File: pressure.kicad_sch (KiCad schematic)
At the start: 7 parts, among them IC1 HSFPAR004A, U6 INA317IDGKR

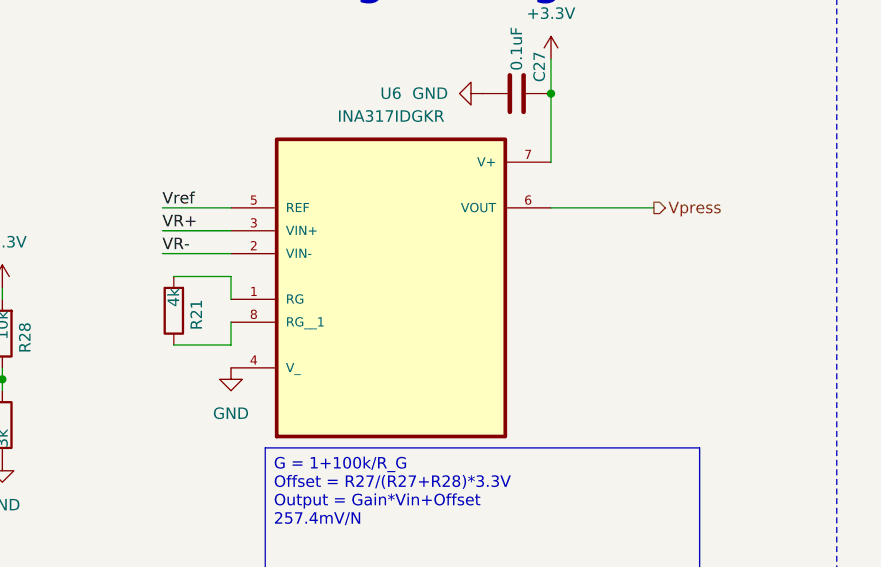
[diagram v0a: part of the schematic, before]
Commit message: further work
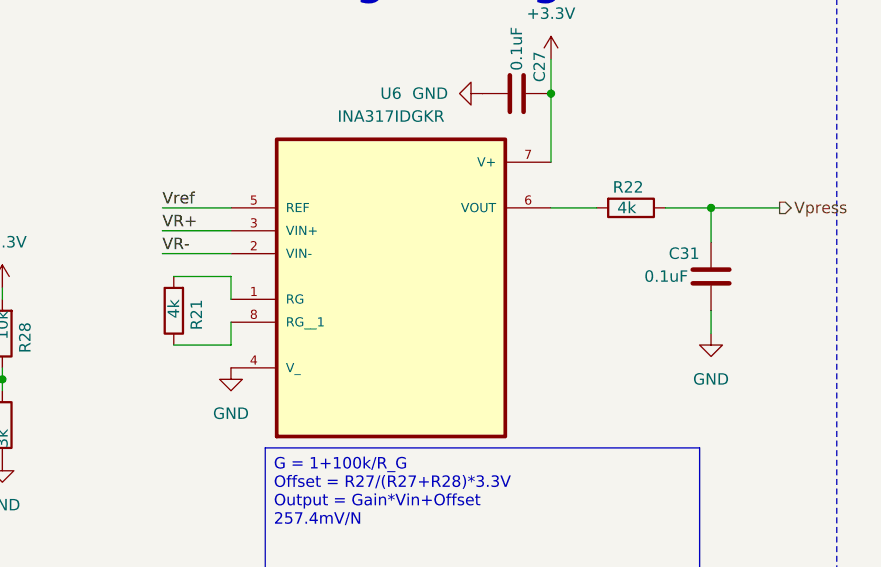
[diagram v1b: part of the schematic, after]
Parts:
- added C31: 0.1uF, Capacitor_SMD:C_0603_1608Metric, symbol Device:C
- added R22: 4k, Resistor_SMD:R_0603_1608Metric, symbol Device:R
- C27, C30: footprint Capacitor_SMD:C_0805_2012Metric -> Capacitor_SMD:C_0603_1608Metric
- R21, R27, R28: footprint Resistor_SMD:R_0805_2012Metric -> Resistor_SMD:R_0603_1608Metric
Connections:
- net GND: now also C31.2
- net Vpress: now also C31.1, R22.1; no longer U6.6 (VOUT)
- new net: R22.2, U6.6 (VOUT)
